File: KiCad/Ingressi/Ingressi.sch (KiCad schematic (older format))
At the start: 4 parts, among them J1 NL4MP-M3, J2 NL4MP-M3, J3 Faston, J4 XXXX

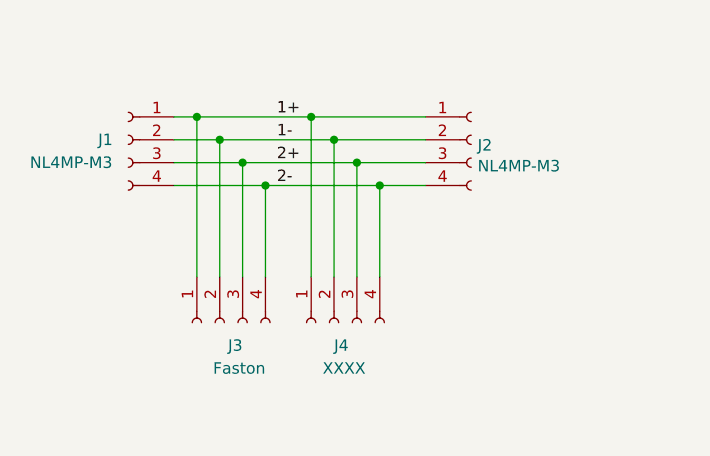
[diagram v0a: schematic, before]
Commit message: schematic finished
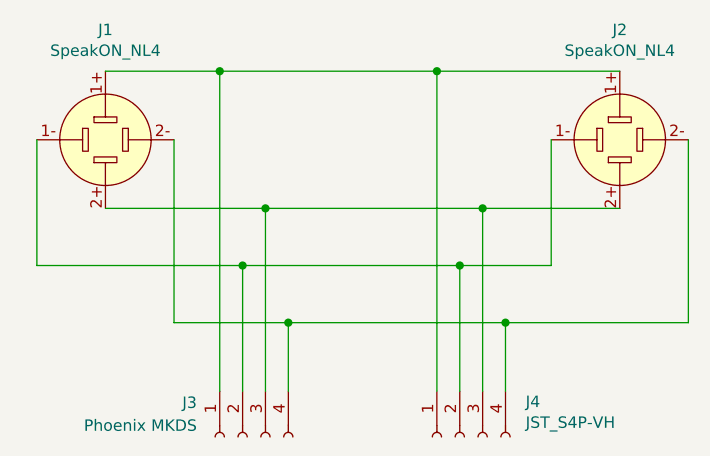
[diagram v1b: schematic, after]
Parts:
- removed J1, J2: NL4MP-M3, symbol Connector:Conn_01x04_Female
- added J1, J2: SpeakON_NL4, Connector Audio:Jack_speakON_Neutrik_NL4MP, symbol Connector:SpeakON_NL4
- J3: value Faston -> Phoenix MKDS; footprint (none) -> Connector Phoenix MSTB:PhoenixContact_MKDS_5_1x04_P6.35mm
- J4: value XXXX -> JST_S4P-VH; footprint (none) -> Connector JST:JST_VH_S4P-VH_1x04_P3.96mm_Horizontal
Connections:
- net 1+: no longer names the net of J3.1 (Pin_1), J4.1 (Pin_1)
- net 1+: now also J1.1+, J2.1+
- net 1-: no longer names the net of J3.2 (Pin_2), J4.2 (Pin_2)
- net 1-: now also J1.1-, J2.1-
- net 2+: no longer names the net of J3.3 (Pin_3), J4.3 (Pin_3)
- net 2+: now also J1.2+, J2.2+
- net 2-: no longer names the net of J3.4 (Pin_4), J4.4 (Pin_4)
- net 2-: now also J1.2-, J2.2-
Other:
- moved on the sheet: J3, J4
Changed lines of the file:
@@
 $EndDescr
 $Comp
-L Connector:Conn_01x04_Female J2
-U 1 1 5FD230A4
-P 6350 3650
-F 0 "J2" H 6378 3626 50  0000 L CNN
-F 1 "NL4MP-M3" H 6378 3535 50  0000 L CNN
-F 2 "" H 6350 3650 50  0001 C CNN
-F 3 "~" H 6350 3650 50  0001 C CNN
-	1    6350 3650
+L Connector:SpeakON_NL4 J1
+U 1 1 5FD43F0D
+P 4750 3650
+F 0 "J1" H 4750 4131 50  0000 C CNN
+F 1 "SpeakON_NL4" H 4750 4040 50  0000 C CNN
+F 2 "Connector Audio:Jack_speakON_Neutrik_NL4MP" H 4750 3650 50  0001 C CNN
+F 3 "http://www.neutrik.com/en/speakon/" H 4750 3650 50  0001 C CNN
+	1    4750 3650
 	1    0    0    -1
 $EndComp
+Wire Wire Line
+	4750 3350 5250 3350
+Wire Wire Line
+	4750 3950 5450 3950
+Wire Wire Line
+	6700 3650 6700 4200
+Wire Wire Line
+	6700 4200 6300 4200
+Wire Wire Line
+	4450 4200 4450 3650
+Wire Wire Line
+	5050 3650 5050 4450
+Wire Wire Line
+	5050 4450 5550 4450
+Wire Wire Line
+	7300 4450 7300 3650
+Wire Wire Line
+	5250 4750 5250 3350
+Connection ~ 5250 3350
+Wire Wire Line
+	5250 3350 6200 3350
+Wire Wire Line
+	5350 4750 5350 4200
+Connection ~ 5350 4200
+Wire Wire Line
+	5350 4200 4450 4200
+Wire Wire Line
+	6200 4750 6200 3350
+Connection ~ 6200 3350
+Wire Wire Line
+	6200 3350 7000 3350
+Wire Wire Line
+	6300 4750 6300 4200
+Connection ~ 6300 4200
+Wire Wire Line
+	6300 4200 5350 4200
+Wire Wire Line
+	5450 4750 5450 3950
+Connection ~ 5450 3950
+Wire Wire Line
+	5450 3950 6400 3950
+Wire Wire Line
+	5550 4750 5550 4450
+Connection ~ 5550 4450
+Wire Wire Line
+	5550 4450 6500 4450
+Wire Wire Line
+	6400 4750 6400 3950
+Connection ~ 6400 3950
+Wire Wire Line
+	6400 3950 7000 3950
+Wire Wire Line
+	6500 4750 6500 4450
+Connection ~ 6500 4450
+Wire Wire Line
+	6500 4450 7300 4450
 $Comp
-L Connector:Conn_01x04_Female J1
-U 1 1 5FD256AD
-P 4850 3650
-F 0 "J1" H 4950 3650 50  0000 C CNN
-F 1 "NL4MP-M3" H 5100 3550 50  0000 C CNN
-F 2 "" H 4850 3650 50  0001 C CNN
-F 3 "~" H 4850 3650 50  0001 C CNN
-	1    4850 3650
-	-1   0    0    -1
+L Connector:SpeakON_NL4 J2
+U 1 1 5FD48C19
+P 7000 3650
+F 0 "J2" H 7000 4131 50  0000 C CNN
+F 1 "SpeakON_NL4" H 7000 4040 50  0000 C CNN
+F 2 "Connector Audio:Jack_speakON_Neutrik_NL4MP" H 7000 3650 50  0001 C CNN
+F 3 "http://www.neutrik.com/en/speakon/" H 7000 3650 50  0001 C CNN
+	1    7000 3650
+	1    0    0    -1
 $EndComp
 $Comp
 L Connector:Conn_01x04_Female J3
 U 1 1 5FD26AE9
-P 5250 4450
-F 0 "J3" V 5350 4350 50  0000 L CNN
-F 1 "Faston" V 5450 4250 50  0000 L CNN
-F 2 "" H 5250 4450 50  0001 C CNN
-F 3 "~" H 5250 4450 50  0001 C CNN
-	1    5250 4450
+P 5350 4950
+F 0 "J3" V 5200 5150 50  0000 L CNN
+F 1 "Phoenix MKDS" V 5300 5150 50  0000 L CNN
+F 2 "Connector Phoenix MSTB:PhoenixContact_MKDS_5_1x04_P6.35mm" H 5350 4950 50  0001 C CNN
+F 3 "~" H 5350 4950 50  0001 C CNN
+	1    5350 4950
 	0    -1   1    0
 $EndComp
@@
 L Connector:Conn_01x04_Female J4
 U 1 1 5FD27467
-P 5750 4450
-F 0 "J4" V 5850 4450 50  0000 R CNN
-F 1 "XXXX" V 5950 4500 50  0000 R CNN
-F 2 "" H 5750 4450 50  0001 C CNN
-F 3 "~" H 5750 4450 50  0001 C CNN
-	1    5750 4450
+P 6300 4950
+F 0 "J4" V 6146 4662 50  0000 R CNN
+F 1 "JST_S4P-VH" V 6237 4662 50  0000 R CNN
+F 2 "Connector JST:JST_VH_S4P-VH_1x04_P3.96mm_Horizontal" H 6300 4950 50  0001 C CNN
+F 3 "~" H 6300 4950 50  0001 C CNN
+	1    6300 4950
 	0    -1   1    0
 $EndComp
-Wire Wire Line
-	5050 3550 5150 3550
-Wire Wire Line
-	5050 3650 5250 3650
-Wire Wire Line
-	5050 3750 5350 3750
-Wire Wire Line
-	5050 3850 5450 3850
-Wire Wire Line
-	5150 4250 5150 3550
-Connection ~ 5150 3550
-Wire Wire Line
-	5150 3550 5650 3550
-Wire Wire Line
-	5250 4250 5250 3650
-Connection ~ 5250 3650
-Wire Wire Line
-	5250 3650 5750 3650
-Wire Wire Line
-	5350 4250 5350 3750
-Connection ~ 5350 3750
-Wire Wire Line
-	5350 3750 5850 3750
-Wire Wire Line
-	5450 4250 5450 3850
-Connection ~ 5450 3850
-Wire Wire Line
-	5450 3850 5950 3850
-Wire Wire Line
-	5650 4250 5650 3550
-Connection ~ 5650 3550
-Wire Wire Line
-	5650 3550 6150 3550
-Wire Wire Line
-	5750 4250 5750 3650
-Connection ~ 5750 3650
-Wire Wire Line
-	5750 3650 6150 3650
-Wire Wire Line
-	5850 4250 5850 3750
-Connection ~ 5850 3750
-Wire Wire Line
-	5850 3750 6150 3750
-Wire Wire Line
-	5950 4250 5950 3850
-Connection ~ 5950 3850
-Wire Wire Line
-	5950 3850 6150 3850
-Text Label 5500 3550 0    50   ~ 0
-1+
-Text Label 5500 3650 0    50   ~ 0
-1-
-Text Label 5500 3750 0    50   ~ 0
-2+
-Text Label 5500 3850 0    50   ~ 0
-2-
 $EndSCHEMATC
